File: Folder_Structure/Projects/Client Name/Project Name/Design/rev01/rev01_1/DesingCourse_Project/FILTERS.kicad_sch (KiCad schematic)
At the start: 17 parts, among them J10 874380643

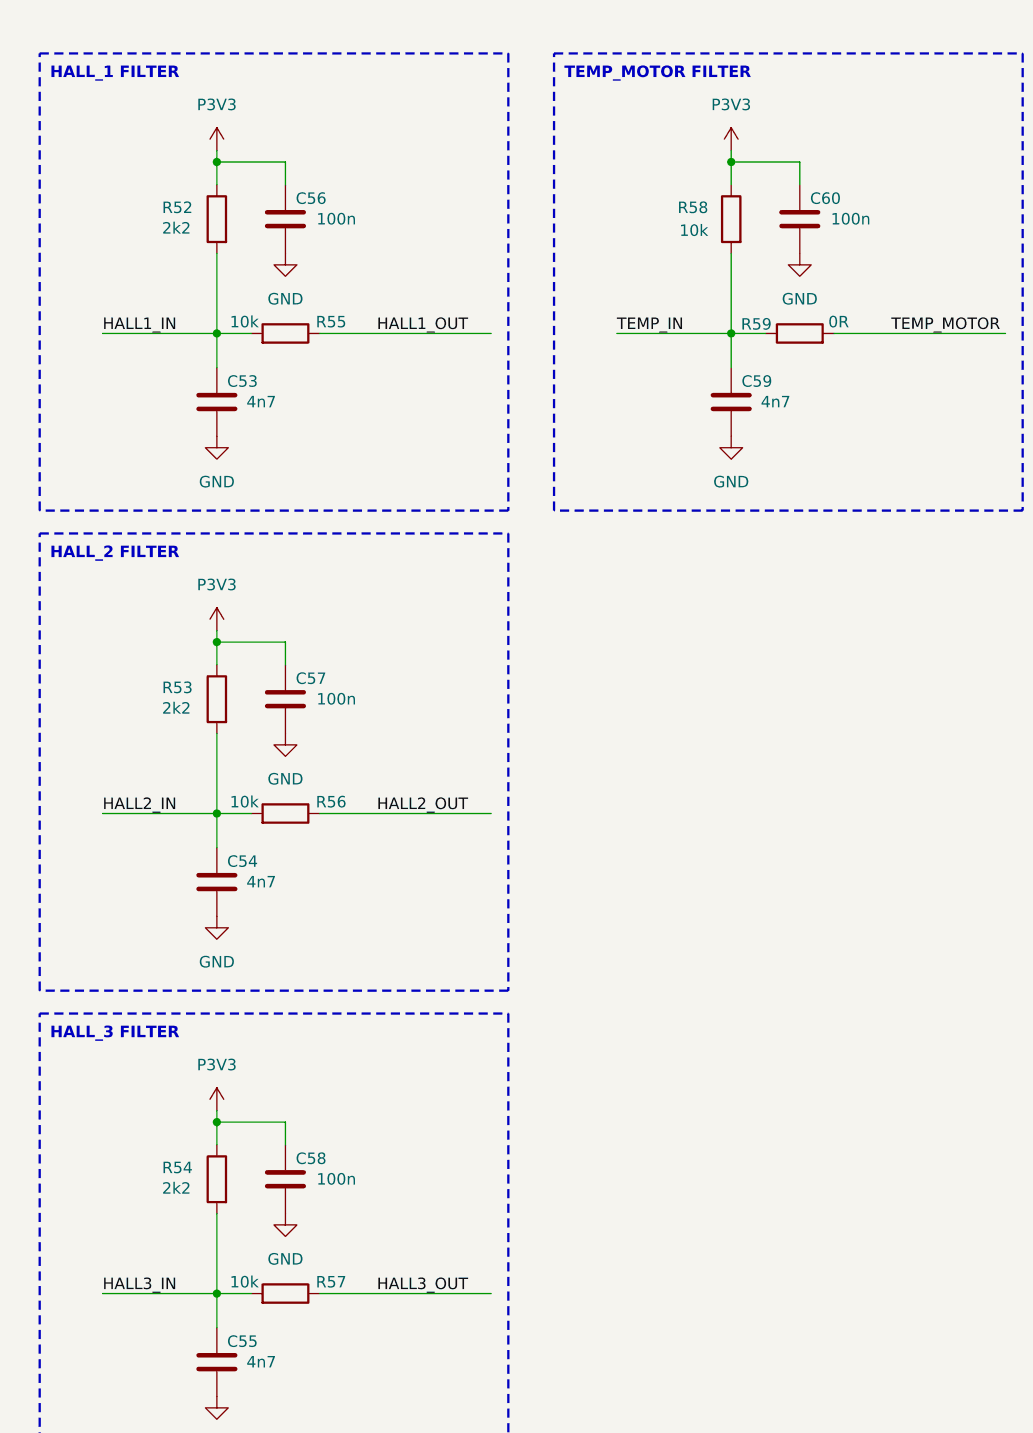
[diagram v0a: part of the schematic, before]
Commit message: Update13
Still working on FP for the MCU
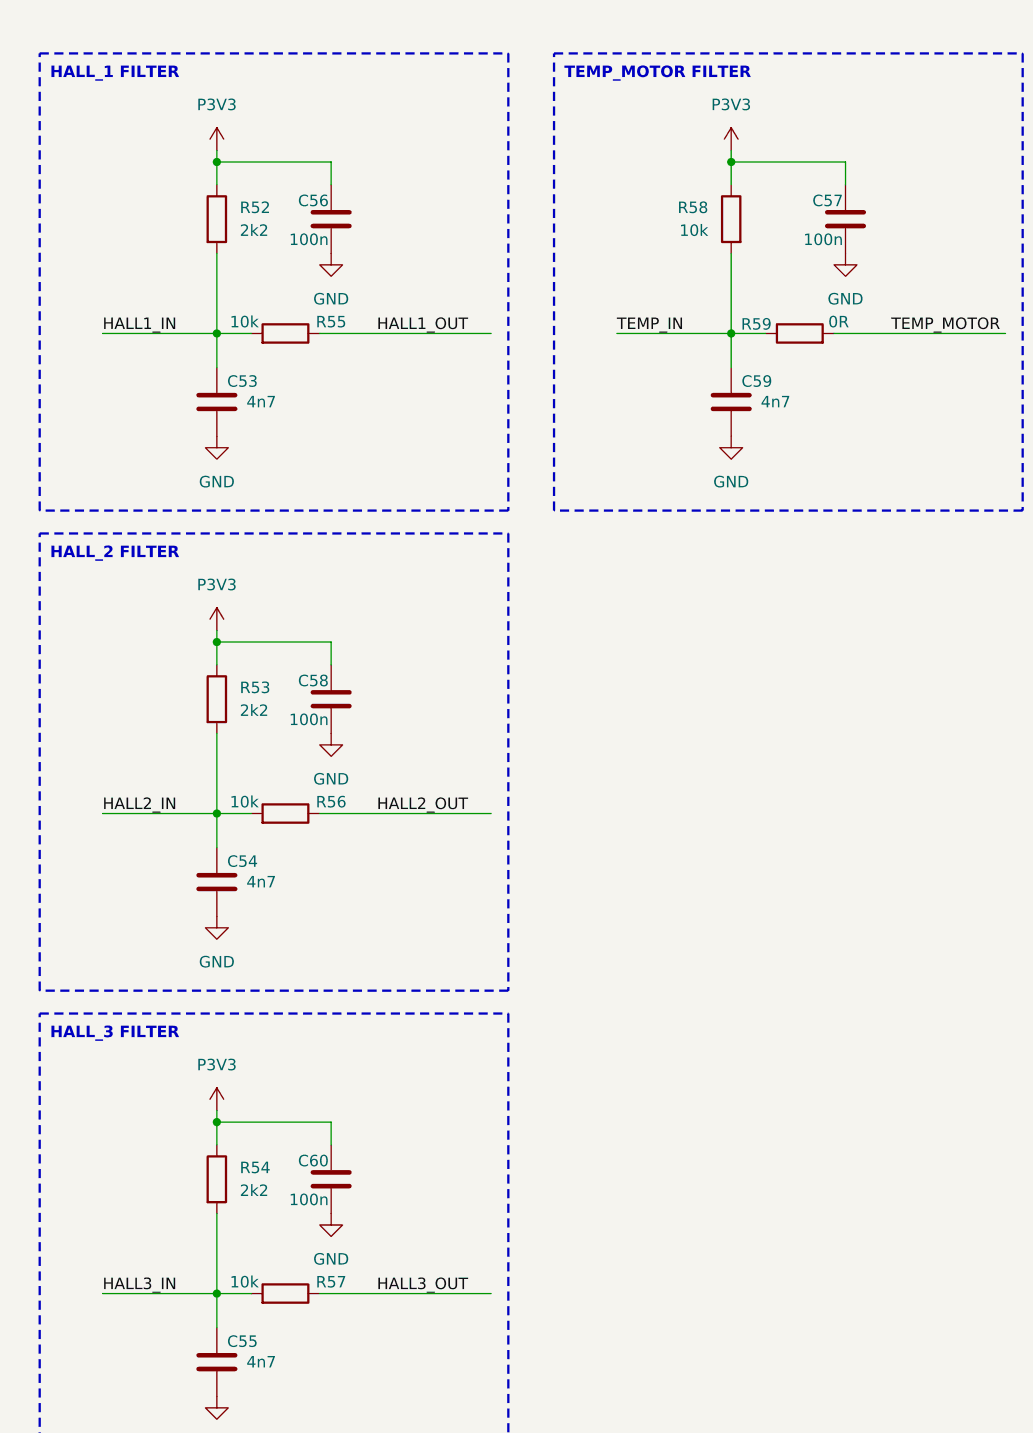
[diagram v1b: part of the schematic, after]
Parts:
- C56, C57, C58, C60: footprint (none) -> Capacitor_SMD:C_0603_1608Metric; Package (none) -> 0603; Temp Coeff (none) -> X7R; Tolerance (none) -> 10%; Voltage Rating (none) -> 10V
- R52, R53, R54: footprint (none) -> Resistor_SMD:R_0603_1608Metric; Package (none) -> 0603; Power Rating (none) -> 1/10W; Tolerance (none) -> 1%
